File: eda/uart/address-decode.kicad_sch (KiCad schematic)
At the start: 5 parts, among them U15 74HCT00, U18 74HCT32, U2 74HCT14, U7 74HCT139

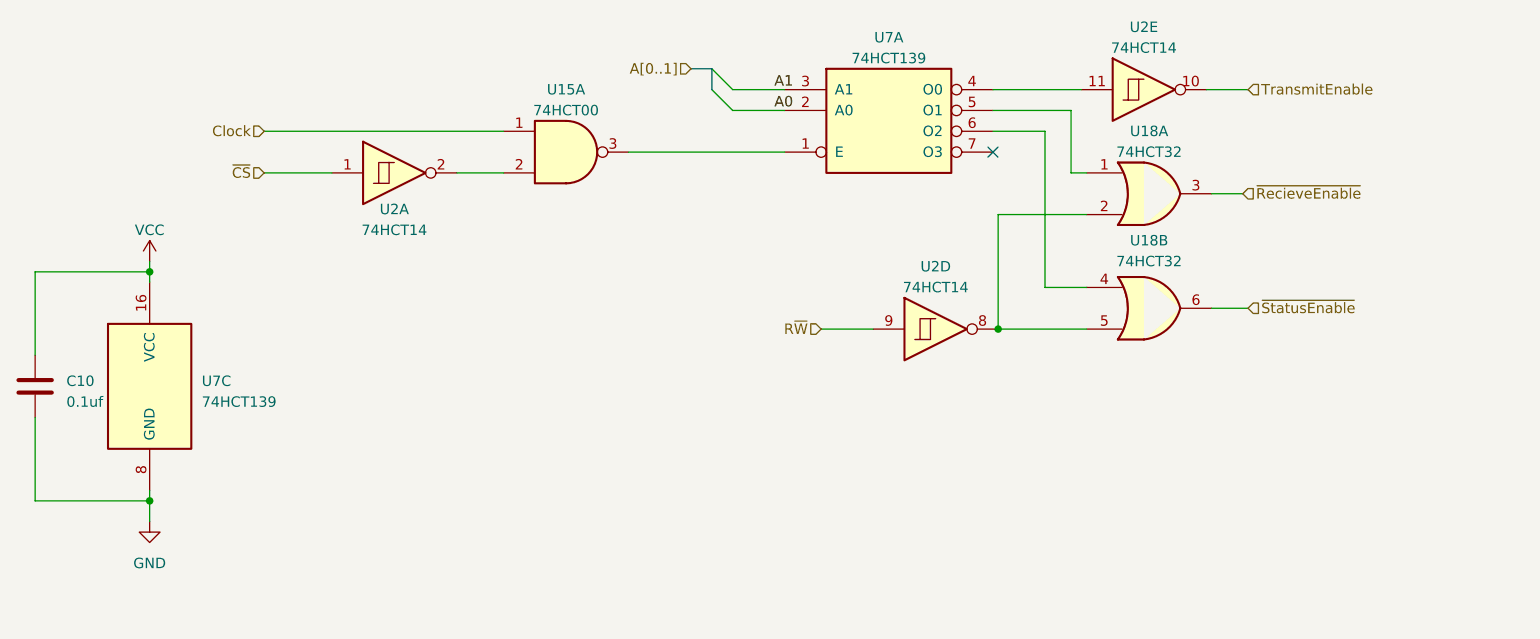
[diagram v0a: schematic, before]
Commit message: Uart eda work
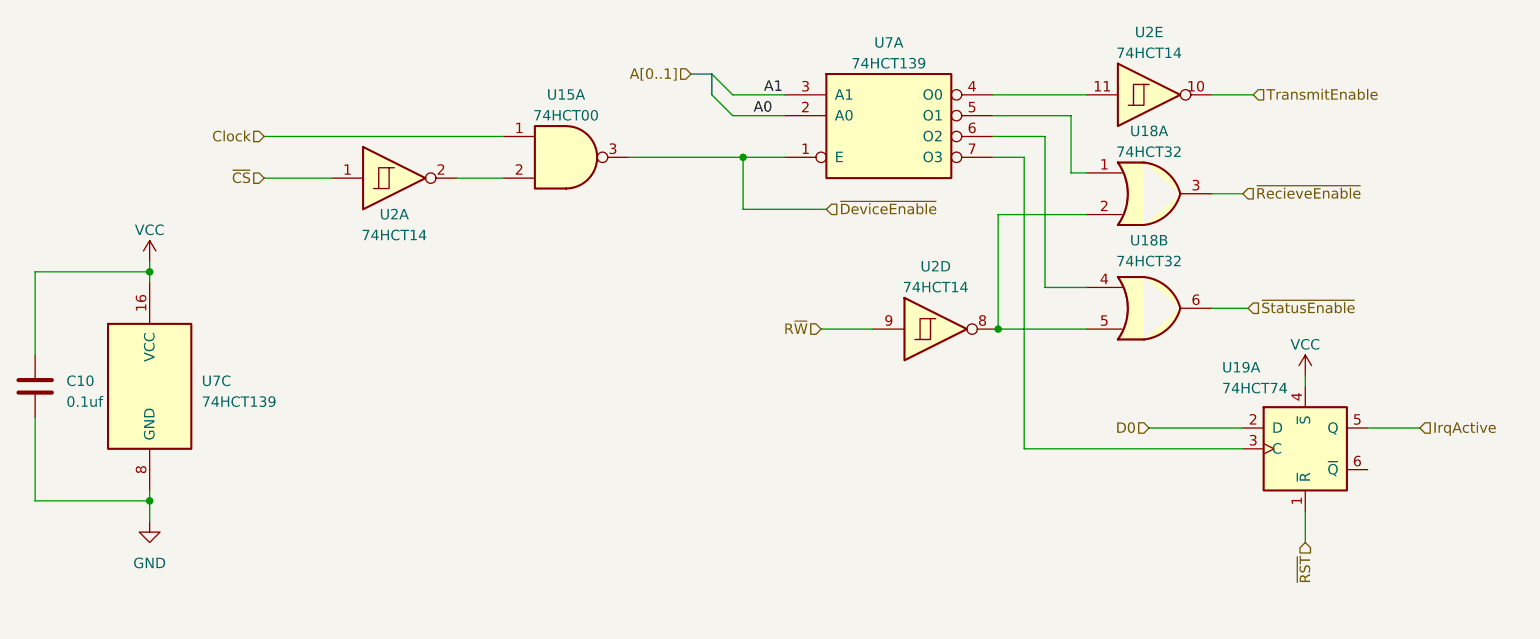
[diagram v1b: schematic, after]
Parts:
- added U19: 74HCT74, Package_DIP:DIP-14_W7.62mm, symbol 74xx:74HC74
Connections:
- net VCC: now also U19.4 (~{S})
- net ~{DeviceEnable}: now reaches U15.3, U7.1 (E)
- net at U7.7 (O3): now also U19.3 (C)
- new net D0: U19.2 (D)
- new net IrqActive: U19.5 (Q)
- new net ~{RST}: U19.1 (~{R})
- no-connect marks 1 -> 0
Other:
- moved on the sheet: U15A, U2A, U2E, U7A
